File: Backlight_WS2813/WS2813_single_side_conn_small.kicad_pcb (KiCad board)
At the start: 2 copper layers, 7.2 x 9.6 mm, 4 parts

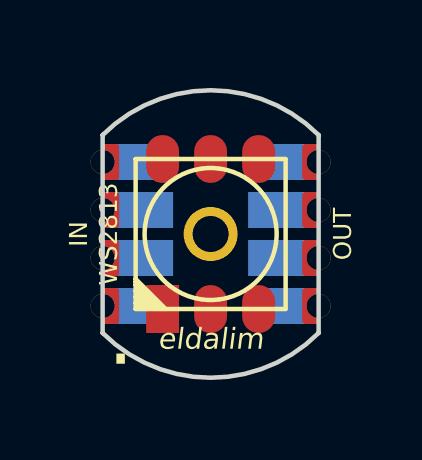
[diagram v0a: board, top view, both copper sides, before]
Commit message: + WS2813_single_side_conn
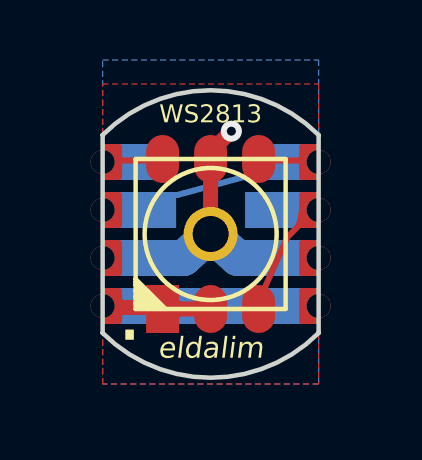
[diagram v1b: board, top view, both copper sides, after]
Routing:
- net GND: track 0.00 -> 9.03 mm, vias 0 -> 1
- net +VCC: track 0.00 -> 8.06 mm
- net /Din: track 0.00 -> 6.55 mm
- net /Dout: track 0.00 -> 3.68 mm
- net /BDin: track 0.00 -> 1.55 mm
- added copper zone on B.Cu, net GND
- added copper zone on F.Cu, net GND
